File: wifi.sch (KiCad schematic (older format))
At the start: 69 parts, among them IC4 WL1835MODGBMOCT, J10 TEST_1P, J11 TEST_1P, J12 ANT2, J13 TEST_1P, J14 TEST_1P, J4 ANT2, J5 TEST_1P, J6 TEST_1P, J7 TEST_1P, J8 TEST_1P, J9 TEST_1P, Q1 BSS138, Q2 BSS138, U10 TXS0108, U11 TXS0108, X1 NZ2520SB-32.768KHZ-NSA3534C

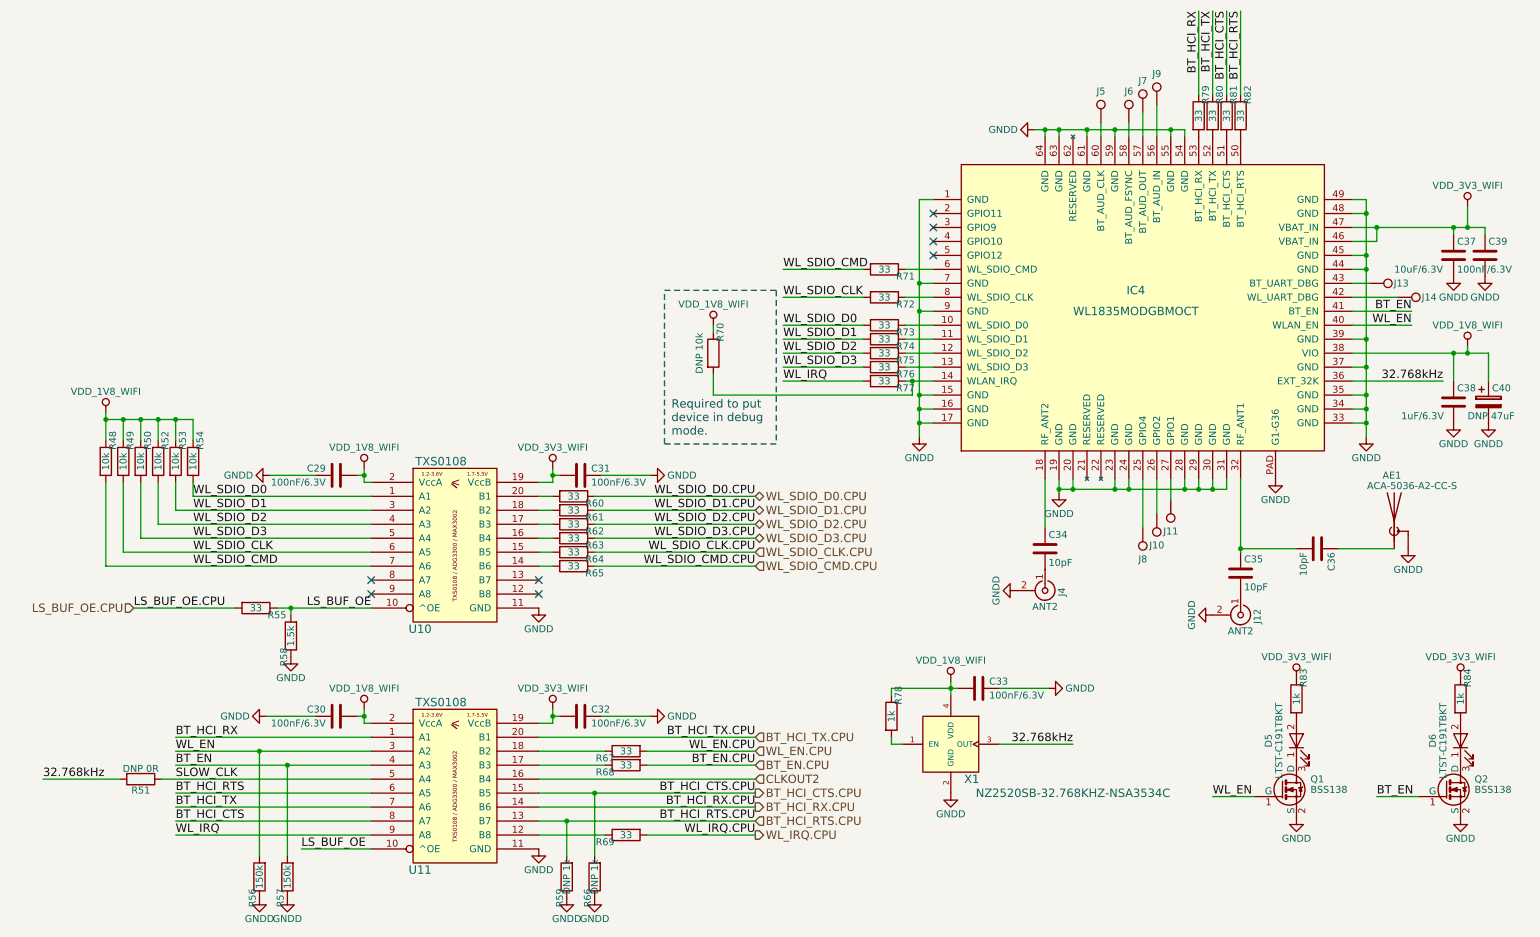
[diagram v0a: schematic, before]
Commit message: wip erc
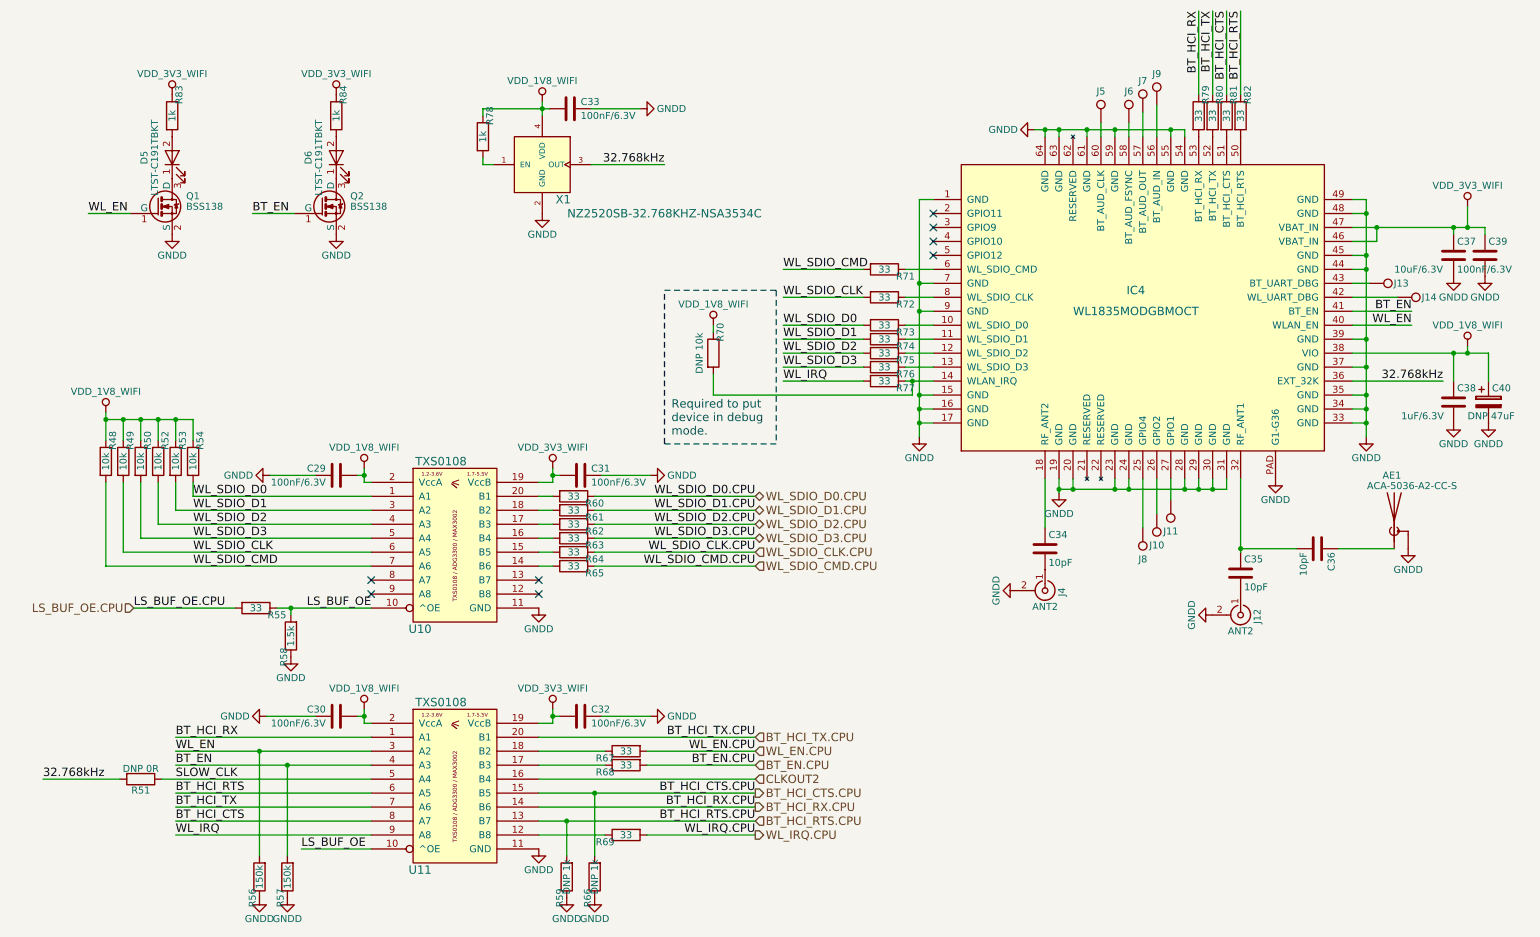
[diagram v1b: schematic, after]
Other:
- moved on the sheet: C33, D5, D6, Q1, Q2, R78, R83, R84, X1

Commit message: wip footprint assoc
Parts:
- C29, C30, C31, C32, C33, C34, C35, C36, C38, C39: footprint (none) -> Capacitors_SMD:C_0402
- C37: footprint (none) -> Capacitors_SMD:C_0603
- C40: footprint (none) -> Capacitors_Tantalum_SMD:CP_Tantalum_Case-A_EIA-3216-18_Reflow
- D5, D6: footprint (none) -> LEDs:LED_0603
- IC4: footprint (none) -> bbblue:BeagleBone_Blue-GHI-IC_MOC-100(TI)
- J10, J11, J13, J14, J5, J6, J7, J8, J9: footprint (none) -> Measurement_Points:Measurement_Point_Round-SMD-Pad_Small
- R48, R49, R50, R51, R52, R53, R54, R55, R56, R57, R58, R59, R60, R61, R62, R63, R64, R65, R66, R67, R68, R69, R70, R71, R72, R73, R74, R75, R76, R77, R78, R79, R80, R81, R82, R83, R84: footprint (none) -> Resistors_SMD:R_0402

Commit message: wip footprint assoc
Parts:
- J12, J4: footprint (none) -> bbblue:BeagleBone_Blue-GHI-CONNECTORS_U.FL-R-SMT-1
- U10, U11: footprint (none) -> Housings_SSOP:TSSOP-20_4.4x6.5mm_Pitch0.65mm
- X1: footprint (none) -> Crystals:Crystal_SMD_2520-4pin_2.5x2.0mm
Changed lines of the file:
@@
 F 0 "U10" H 3350 3775 60  0000 C CNN
 F 1 "TXS0108" H 3500 4975 60  0000 C CNN
-F 2 "" H 3600 4375 60  0001 C CNN
+F 2 "Housings_SSOP:TSSOP-20_4.4x6.5mm_Pitch0.65mm" H 3600 4375 60  0001 C CNN
 F 3 "" H 3600 4375 60  0001 C CNN
 	1    3600 4375
@@
 F 0 "U11" H 3350 5500 60  0000 C CNN
 F 1 "TXS0108" H 3500 6700 60  0000 C CNN
-F 2 "" H 3600 6100 60  0001 C CNN
+F 2 "Housings_SSOP:TSSOP-20_4.4x6.5mm_Pitch0.65mm" H 3600 6100 60  0001 C CNN
 F 3 "" H 3600 6100 60  0001 C CNN
 	1    3600 6100
@@
 F 0 "J4" H 7835 4820 50  0000 C CNN
 F 1 "ANT2" V 7940 4700 50  0000 C CNN
-F 2 "" H 7825 4700 50  0001 C CNN
+F 2 "bbblue:BeagleBone_Blue-GHI-CONNECTORS_U.FL-R-SMT-1" H 7825 4700 50  0001 C CNN
 F 3 "" H 7825 4700 50  0001 C CNN
 	1    7825 4700
@@
 F 0 "J12" H 9235 4995 50  0000 C CNN
 F 1 "ANT2" V 9340 4875 50  0000 C CNN
-F 2 "" H 9225 4875 50  0001 C CNN
+F 2 "bbblue:BeagleBone_Blue-GHI-CONNECTORS_U.FL-R-SMT-1" H 9225 4875 50  0001 C CNN
 F 3 "" H 9225 4875 50  0001 C CNN
 	1    9225 4875
@@
 F 0 "X1" H 4375 1400 60  0000 C CNN
 F 1 "NZ2520SB-32.768KHZ-NSA3534C" H 5100 1300 60  0000 C CNN
-F 2 "" H 4225 1650 60  0001 C CNN
+F 2 "Crystals:Crystal_SMD_2520-4pin_2.5x2.0mm" H 4225 1650 60  0001 C CNN
 F 3 "" H 4225 1650 60  0001 C CNN
 	1    4225 1650
